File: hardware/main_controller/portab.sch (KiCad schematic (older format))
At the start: 2 parts

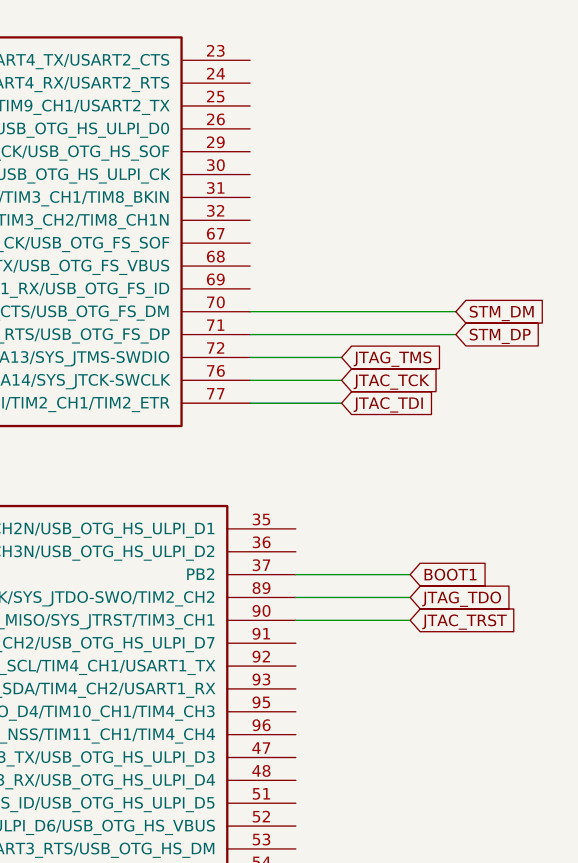
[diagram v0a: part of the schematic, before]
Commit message: Peripherals
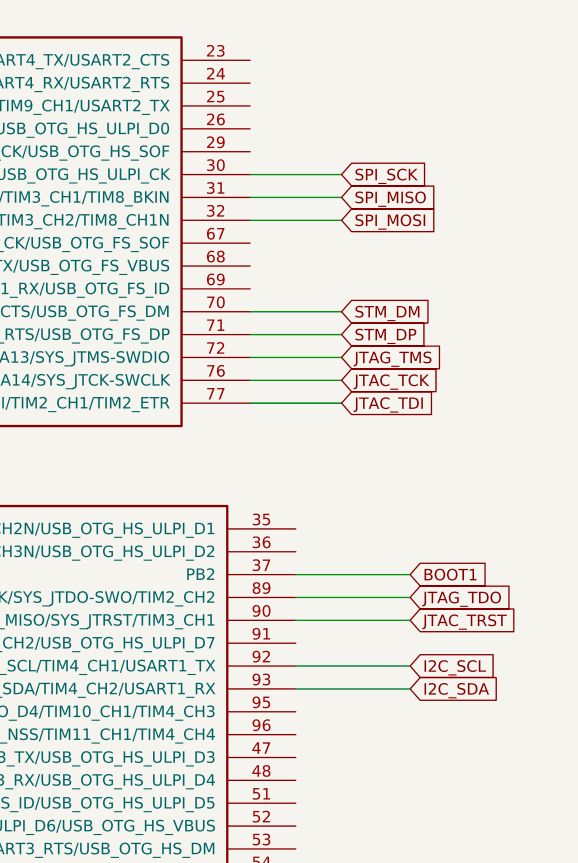
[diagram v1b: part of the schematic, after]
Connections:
- net SPI_SCK: now reaches U?.30 (PA5/ADC1_IN5/ADC2_IN5/DAC_OUT2/SPI1_SCK/TIM2_CH1/TIM2_ETR/TIM8_CH1N/USB_OTG_HS_ULPI_CK)
- net SPI_MISO: now reaches U?.31 (PA6/ADC1_IN6/ADC2_IN6/DCMI_PIXCK/SPI1_MISO/TIM13_CH1/TIM1_BKIN/TIM3_CH1/TIM8_BKIN)
- net SPI_MOSI: now reaches U?.32 (PA7/ADC1_IN7/ADC2_IN7/ETH_CRS_DV/ETH_RX_DV/SPI1_MOSI/TIM14_CH1/TIM1_CH1N/TIM3_CH2/TIM8_CH1N)
- net I2C_SCL: now reaches U?.92 (PB6/CAN2_TX/DCMI_D5/I2C1_SCL/TIM4_CH1/USART1_TX)
- net I2C_SDA: now reaches U?.93 (PB7/DCMI_VSYNC/FSMC_NL/I2C1_SDA/TIM4_CH2/USART1_RX)
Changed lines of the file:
@@
 	1    0    0    -1
 $EndComp
-Wire Wire Line
-	6100 2300 7000 2300
-Wire Wire Line
-	6100 2400 7000 2400
-Text GLabel 7000 2300 2    50   Input ~ 0
+Text GLabel 6500 2300 2    50   Input ~ 0
 STM_DM
-Text GLabel 7000 2400 2    50   Input ~ 0
+Text GLabel 6500 2400 2    50   Input ~ 0
 STM_DP
 $Comp
@@
 Text GLabel 6800 3450 2    50   Input ~ 0
 BOOT1
+Wire Wire Line
+	6300 3850 6800 3850
+Wire Wire Line
+	6300 3950 6800 3950
+Text GLabel 6800 3850 2    50   Input ~ 0
+I2C_SCL
+Text GLabel 6800 3950 2    50   Input ~ 0
+I2C_SDA
+Wire Wire Line
+	6100 1700 6500 1700
+Wire Wire Line
+	6100 1800 6500 1800
+Wire Wire Line
+	6500 1900 6100 1900
+Text GLabel 6500 1700 2    50   Input ~ 0
+SPI_SCK
+Text GLabel 6500 1800 2    50   Input ~ 0
+SPI_MISO
+Text GLabel 6500 1900 2    50   Input ~ 0
+SPI_MOSI
+Wire Wire Line
+	6500 2300 6100 2300
+Wire Wire Line
+	6100 2400 6500 2400
 $EndSCHEMATC

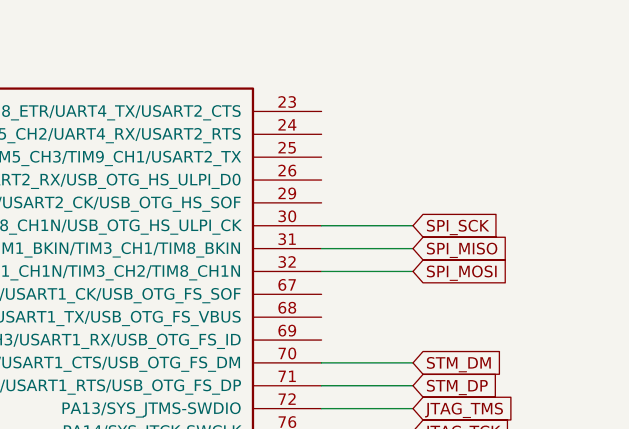
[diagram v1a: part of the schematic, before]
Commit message: LEDs
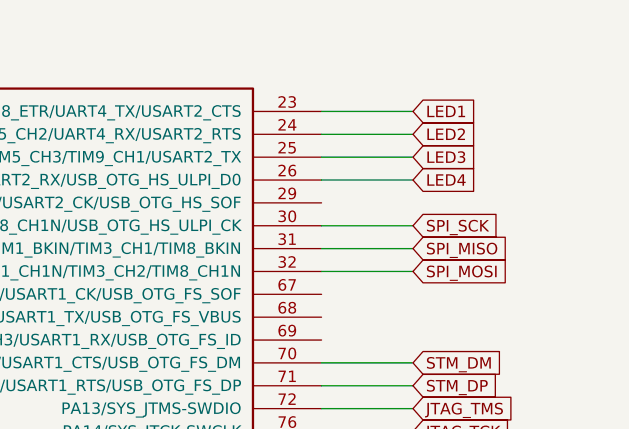
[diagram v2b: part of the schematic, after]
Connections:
- net LED1: now reaches U?.23 (PA0-WKUP/ADC1_IN0/ADC2_IN0/ADC3_IN0/ETH_CRS/SYS_WKUP/TIM2_CH1/TIM2_ETR/TIM5_CH1/TIM8_ETR/UART4_TX/USART2_CTS)
- net LED2: now reaches U?.24 (PA1/ADC1_IN1/ADC2_IN1/ADC3_IN1/ETH_REF_CLK/ETH_RX_CLK/TIM2_CH2/TIM5_CH2/UART4_RX/USART2_RTS)
- net LED3: now reaches U?.25 (PA2/ADC1_IN2/ADC2_IN2/ADC3_IN2/ETH_MDIO/TIM2_CH3/TIM5_CH3/TIM9_CH1/USART2_TX)
- net LED4: now reaches U?.26 (PA3/ADC1_IN3/ADC2_IN3/ADC3_IN3/ETH_COL/TIM2_CH4/TIM5_CH4/TIM9_CH2/USART2_RX/USB_OTG_HS_ULPI_D0)
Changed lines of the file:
@@
 Wire Wire Line
 	6100 2400 6500 2400
+Wire Wire Line
+	6100 1200 6500 1200
+Wire Wire Line
+	6100 1300 6500 1300
+Wire Wire Line
+	6100 1400 6500 1400
+Wire Wire Line
+	6100 1500 6500 1500
+Text GLabel 6500 1200 2    50   Input ~ 0
+LED1
+Text GLabel 6500 1300 2    50   Input ~ 0
+LED2
+Text GLabel 6500 1400 2    50   Input ~ 0
+LED3
+Text GLabel 6500 1500 2    50   Input ~ 0
+LED4
 $EndSCHEMATC
